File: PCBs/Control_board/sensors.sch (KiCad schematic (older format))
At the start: 16 parts, among them J11 Conn_01x02_Male, J12 Conn_01x02_Male, J14 Conn_01x03_Male, J15 Conn_01x02_Male, Q3 PMOS, Q6 Q_NMOS_GSD, SW1 SW_DPST

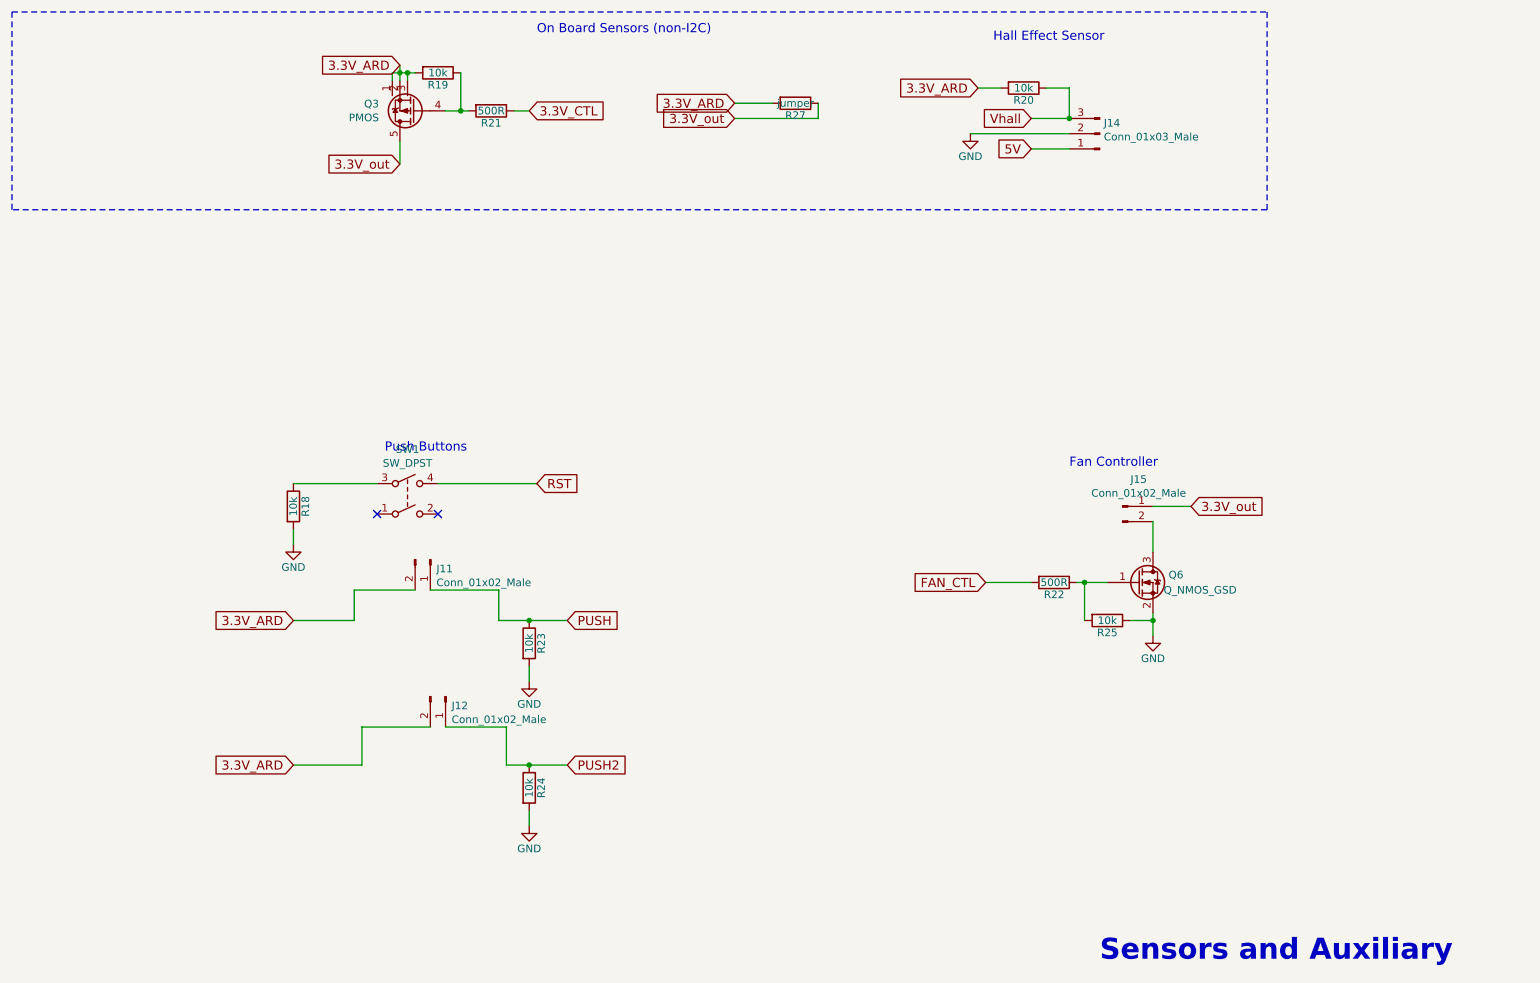
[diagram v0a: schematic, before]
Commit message: Update for revision05a
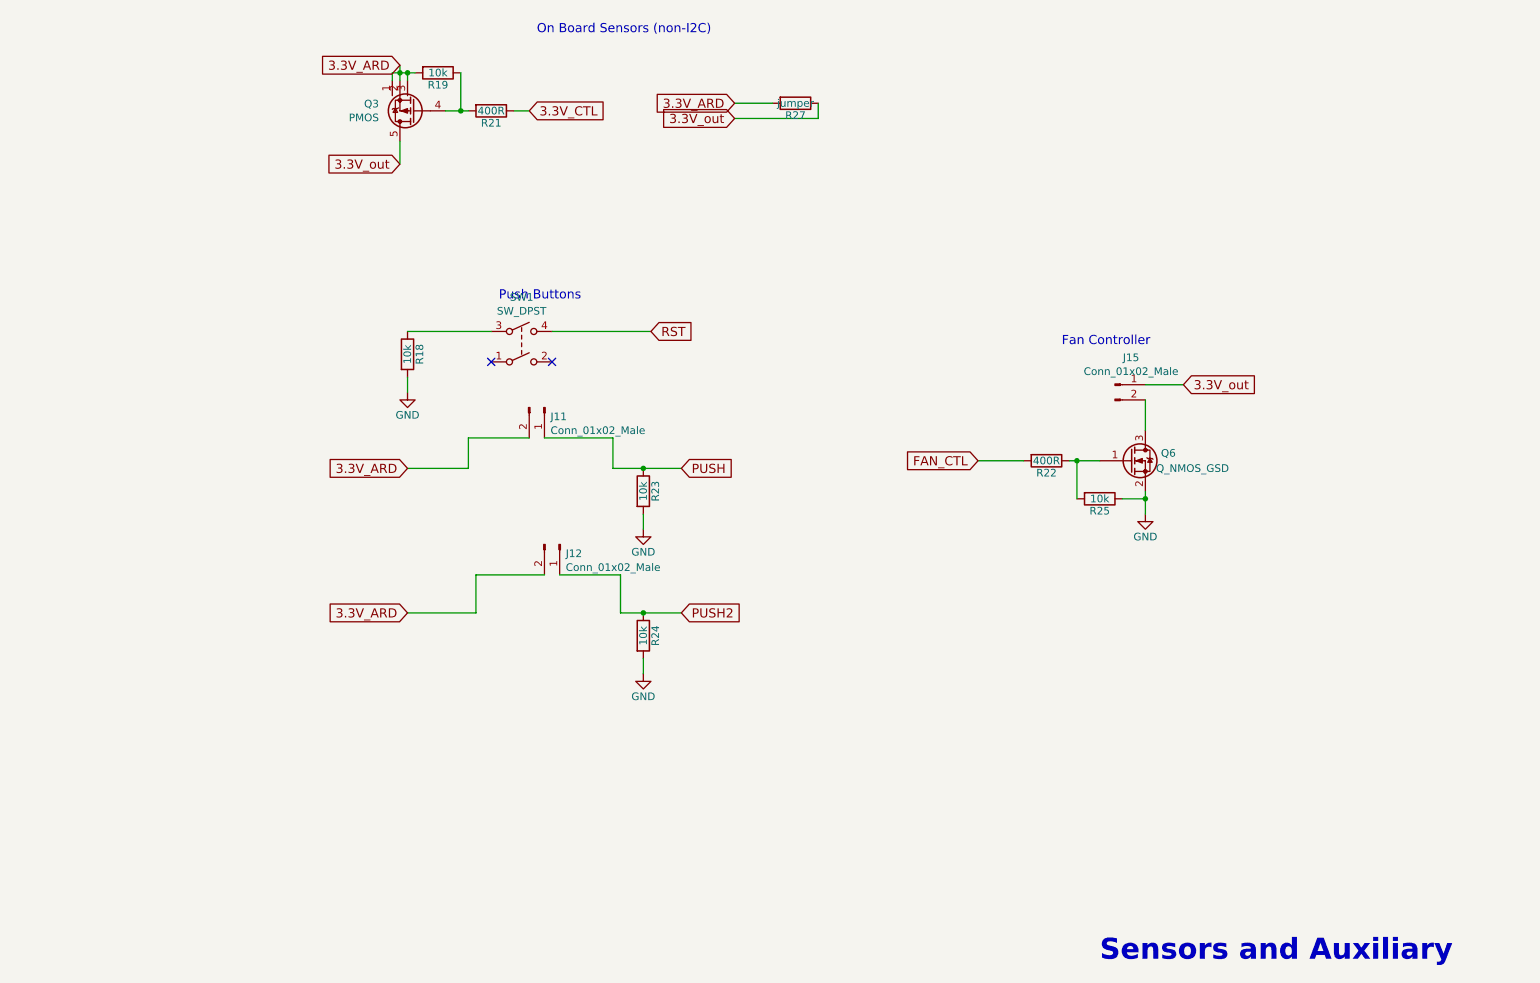
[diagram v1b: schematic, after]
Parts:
- removed J14: Conn_01x03_Male, Connector_JST:JST_PH_B3B-PH-K_1x03_P2.00mm_Vertical, symbol Connector:Conn_01x03_Male
- removed R20: 10k, Resistor_SMD:R_0603_1608Metric, symbol Device:R
- Q6: LCSC (none) -> C382335
- R18, R19, R23, R24, R25: LCSC (none) -> C25804
- R21, R22: value 500R -> 400R; LCSC (none) -> C23193
- SW1: LCSC (none) -> C318888
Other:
- note removed: "Hall Effect Sensor"
- moved on the sheet: J11, J12, J15, Q6, R18, R22, R23, R24, R25, SW1
